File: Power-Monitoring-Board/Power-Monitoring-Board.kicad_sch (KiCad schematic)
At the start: 43 parts, among them IC1 XC6222D331MR-G, J1 Conn_01x02_Pin, J2 Conn_01x02_Pin, J3 Conn_01x01_Pin, J4 Conn_01x01_Pin, J5 Conn_01x01_Pin, J6 Conn_01x01_Pin, J7 Conn_01x02_Pin, J8 Conn_01x02_Pin, SW1 GF-123-0054, U1 INA260AIPWR, U2 CR2450, U3 MAX17043G+U, U4 NUCLEO_L432KC, U5 ST7735R

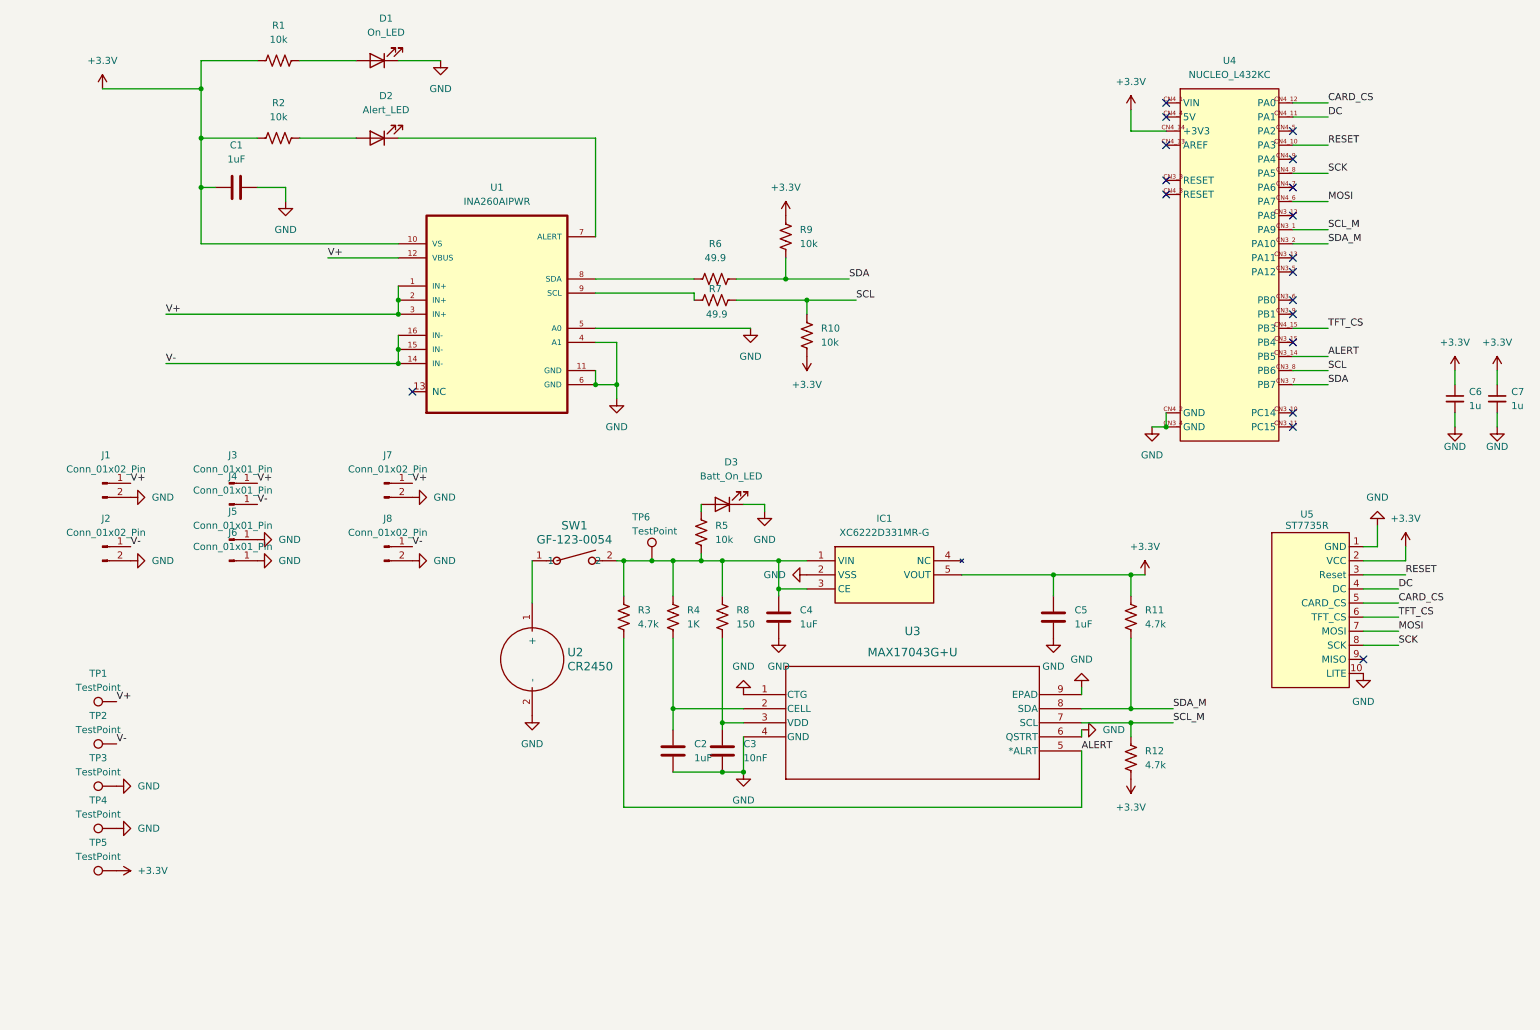
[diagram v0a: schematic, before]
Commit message: changes
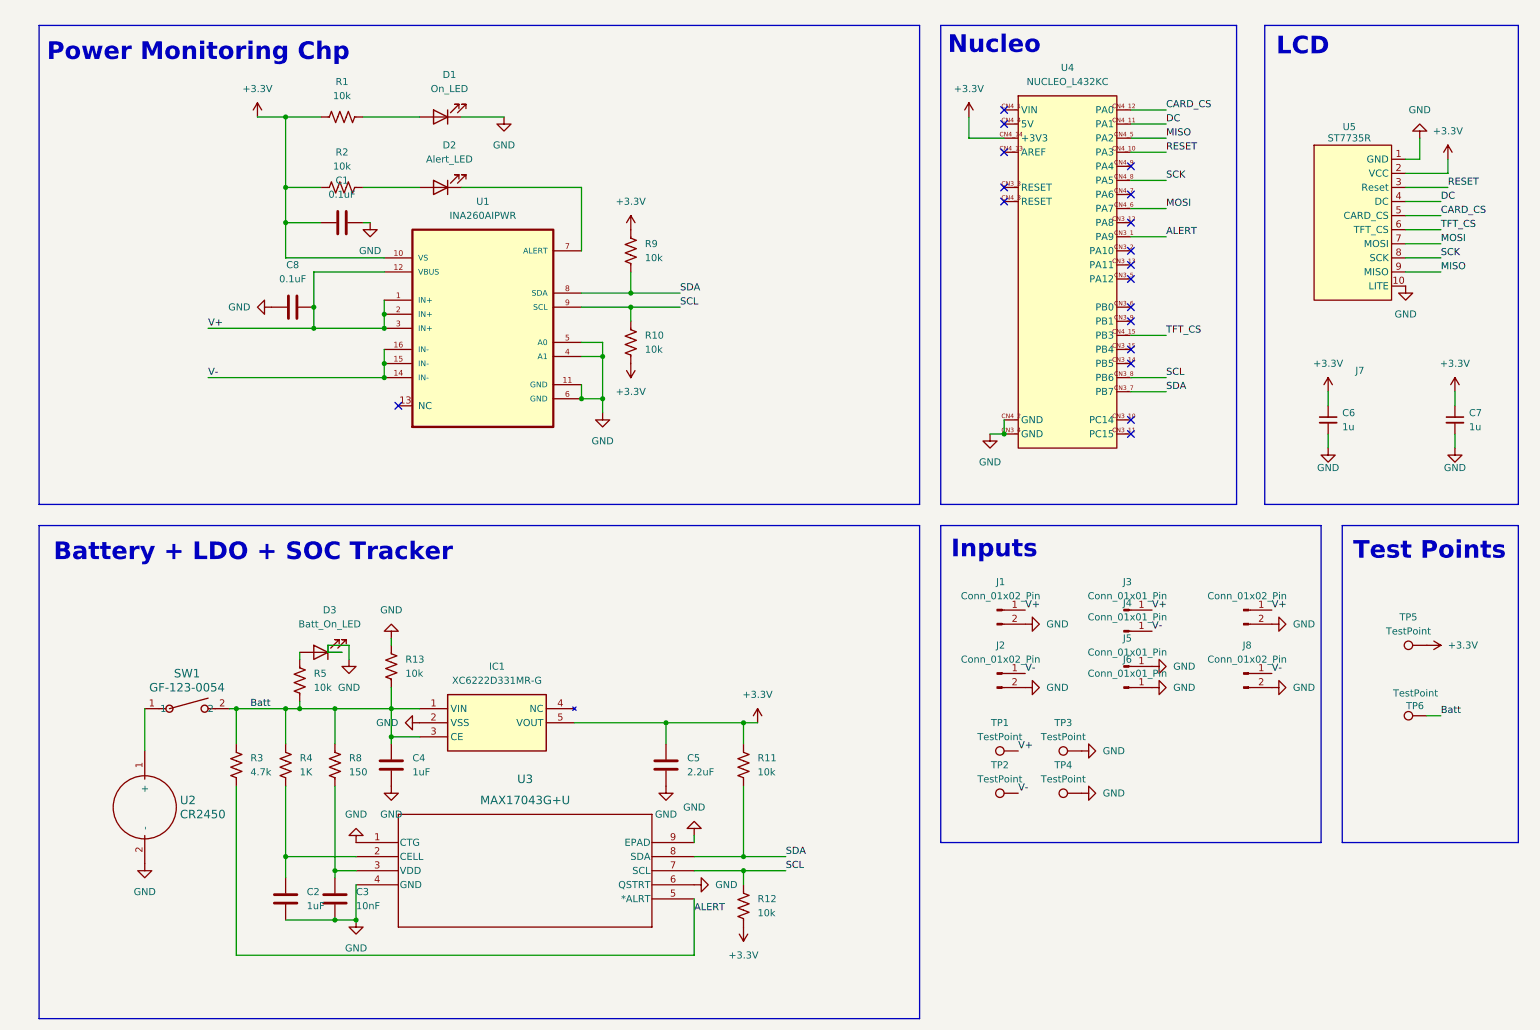
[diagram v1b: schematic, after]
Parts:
- removed R6, R7: 49.9, Resistor_SMD:R_0805_2012Metric, symbol Device:R_US
- added C8: 0.1uF, Capacitor_SMD:C_0805_2012Metric, symbol Device:C
- added R13: 10k, Resistor_SMD:R_0805_2012Metric, symbol Device:R_US
- C1: value 1uF -> 0.1uF
- C5: value 1uF -> 2.2uF
- R11, R12: value 4.7k -> 10k
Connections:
- net ALERT: now also U4.CN3_1 (PA9); no longer U4.CN3_14 (PB5)
- net GND: now also C8.1, R13.1
- net SCL: now also R12.2, U1.9 (SCL), U3.7 (SCL)
- net SDA: now also R11.2, U1.8 (SDA), U3.8 (SDA)
- net V+: now also C8.2
- net Batt: now reaches C4.2, IC1.1 (VIN), IC1.3 (CE), R3.1, R4.1, R5.2, R8.1, SW1.2, TP6.1
- net Batt: now also R13.2
- net MISO: now reaches U5.9 (MISO)
- net MISO: now also U4.CN4_5 (PA2)
- removed net SCL_M: R12.2, U3.7 (SCL), U4.CN3_1 (PA9)
- removed net SDA_M: R11.2, U3.8 (SDA), U4.CN3_2 (PA10)
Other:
- note added: "Battery + LDO + SOC Tracker"
- note added: "Inputs"
- note added: "LCD"
- note added: "Nucleo"
- note added: "Power Monitoring Chp"
- note added: "Test Points"
- moved on the sheet: C1, C2, C3, C4, C5, C6, C7, D1, D2, D3, IC1, J1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
